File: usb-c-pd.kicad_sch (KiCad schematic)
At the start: 18 parts, among them J10 Conn_01x04_Pin, J11 USB_C_Receptacle_USB2.0_16P, J12 Conn_01x03_Pin, J6 Conn_01x02_Socket, Q4 AO3400A, U6 IP2721

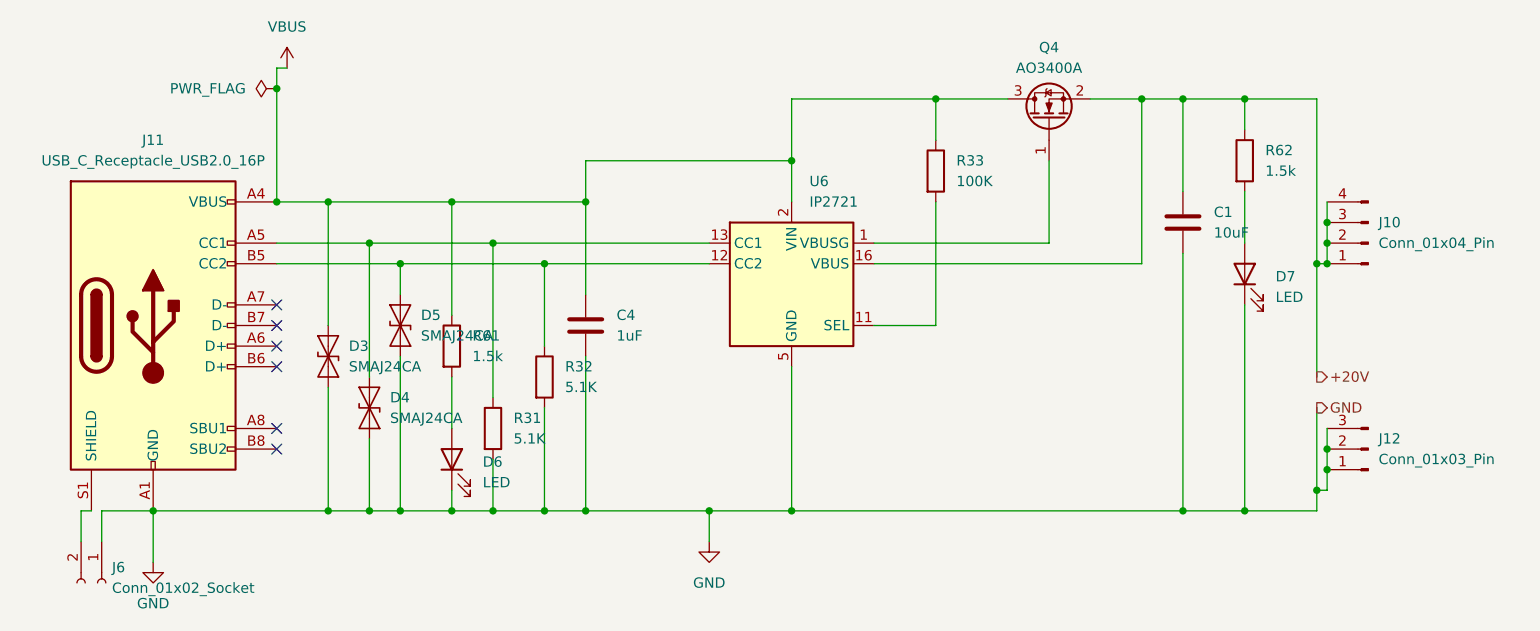
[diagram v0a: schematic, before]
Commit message: change some last parts.
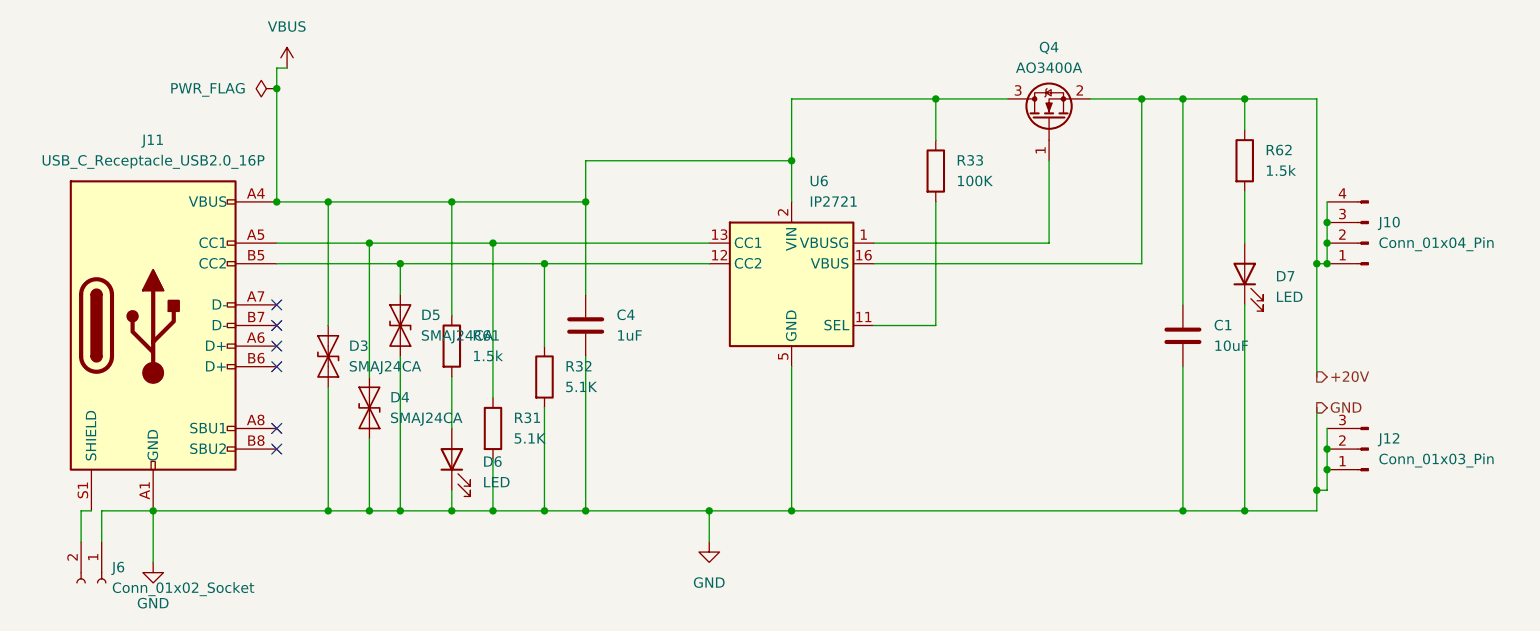
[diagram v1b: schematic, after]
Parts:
- Q4: LCSC (none) -> C20917
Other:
- moved on the sheet: C1
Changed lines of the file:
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@@
 	(wire
 		(pts
-			(xy 167.64 58.42) (xy 167.64 46.99)
+			(xy 167.64 72.39) (xy 167.64 46.99)
 		)
 		(stroke
@@
 	(wire
 		(pts
-			(xy 167.64 66.04) (xy 167.64 97.79)
+			(xy 167.64 80.01) (xy 167.64 97.79)
 		)
 		(stroke
@@
 	(symbol
 		(lib_id "Device:C")
-		(at 167.64 62.23 0)
+		(at 167.64 76.2 0)
 		(unit 1)
 		(exclude_from_sim no)
@@
 		(dnp no)
 		(property "Reference" "C1"
-			(at 171.45 60.9599 0)
+			(at 171.45 74.9299 0)
 			(effects
 				(font
@@
 		)
 		(property "Value" "10uF"
-			(at 171.45 63.4999 0)
+			(at 171.45 77.4699 0)
 			(effects
 				(font
@@
 		)
 		(property "Footprint" "Capacitor_SMD:C_0603_1608Metric"
-			(at 168.6052 66.04 0)
+			(at 168.6052 80.01 0)
 			(effects
 				(font
@@
 		)
 		(property "Datasheet" "~"
-			(at 167.64 62.23 0)
+			(at 167.64 76.2 0)
 			(effects
 				(font
@@
 		)
 		(property "Description" "Unpolarized capacitor"
-			(at 167.64 62.23 0)
+			(at 167.64 76.2 0)
 			(effects
 				(font
@@
 			(effects
 				(font
+					(size 1.27 1.27)
+				)
+				(hide yes)
+			)
+		)
+		(property "LCSC" "C20917"
+			(at 151.13 49.53 90)
+			(effects
+				(font
